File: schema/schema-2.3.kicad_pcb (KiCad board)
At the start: 2 copper layers, 91.4 x 55.9 mm, 16 parts, among them J1 Conn_01x04_Male, J2 Conn_01x04_Male, J3 Conn_01x05_Male

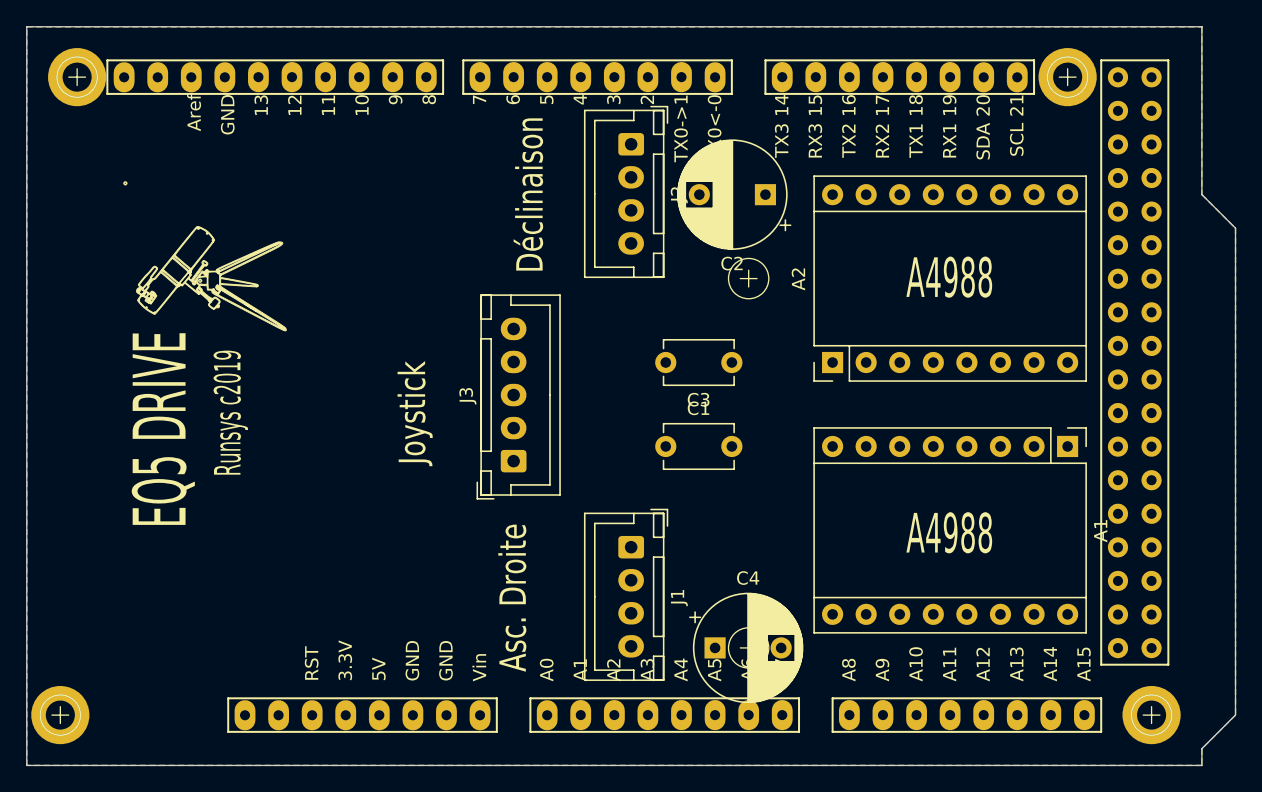
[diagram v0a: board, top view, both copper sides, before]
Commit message: Nouvelle version Version  : 1.0 2.0 2.2 2.3
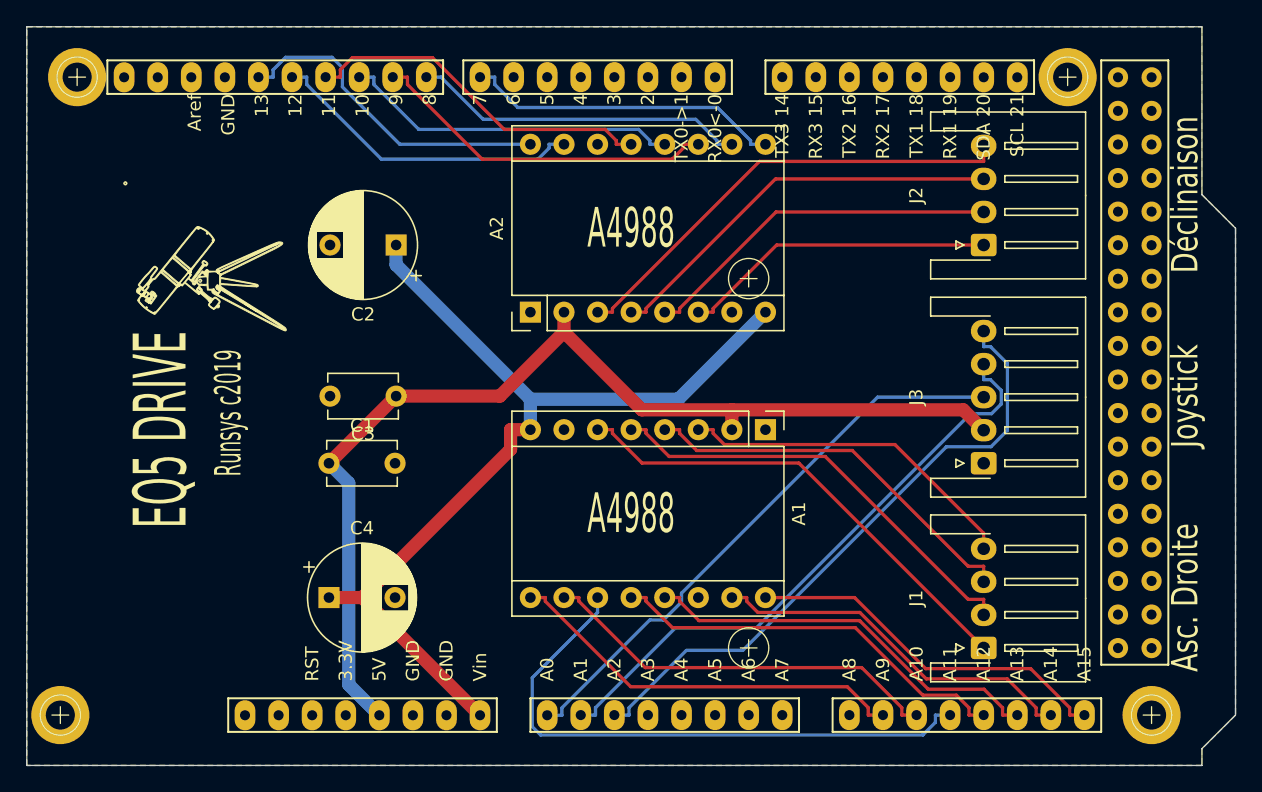
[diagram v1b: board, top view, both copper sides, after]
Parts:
- J1, J2: footprint Connector_JST:JST_XH_B4B-XH-A_1x04_P2.50mm_Vertical -> Connector_JST:JST_XH_S4B-XH-A-1_1x04_P2.50mm_Horizontal
- J3: footprint Connector_JST:JST_XH_B5B-XH-A_1x05_P2.50mm_Vertical -> Connector_JST:JST_XH_S5B-XH-A-1_1x05_P2.50mm_Horizontal
- moved J3 35.6 mm to (163.8, 95.2)
- moved C4 29.5 mm to (114.3, 105.4)
- moved C2 28.2 mm to (119.4, 78.7)
- moved J1 27.7 mm to (163.8, 109.2), turned to 90 degrees
- moved J2 27.7 mm to (163.8, 78.7), turned to 90 degrees
- moved C3 25.5 mm to (119.4, 90.2)
- moved C1 25.5 mm to (114.3, 95.2)
- moved A2 23.2 mm to (129.5, 83.8)
- moved A1 22.9 mm to (147.3, 92.7)
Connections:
- net Net-(J3-Pad3) renamed /A0
- net Net-(J3-Pad4) renamed /A1
- J3 pad 5: Net-(J3-Pad5) -> /A2
- SH1 pad 2: Net-(J3-Pad5) -> Net-(SH1-Pad2)
- SH1 pad A2: Net-(SH1-PadA2) -> /A2
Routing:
- net +5V: track 0.00 -> 80.4 mm
- net +12V: track 0.00 -> 72.6 mm
- net /A2: track 0.00 -> 47.5 mm
- net /A1: track 0.00 -> 45.7 mm
- net /A11: track 0.00 -> 44.6 mm
- net /A0: track 0.00 -> 43.7 mm
- net Net-(A1-Pad6): track 0.00 -> 36.2 mm
- net Net-(A2-Pad3): track 0.00 -> 35.3 mm
- net Net-(A1-Pad5): track 0.00 -> 33.3 mm
- net Net-(A2-Pad4): track 0.00 -> 31.0 mm
- net /A9: track 0.00 -> 30.8 mm
- net /A13: track 0.00 -> 30.8 mm
- net /A12: track 0.00 -> 30.8 mm
- net /A10: track 0.00 -> 30.8 mm
- net Net-(A1-Pad4): track 0.00 -> 29.8 mm
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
